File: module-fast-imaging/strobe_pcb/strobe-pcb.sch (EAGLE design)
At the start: 7 parts, among them IC2 PIC16F18857

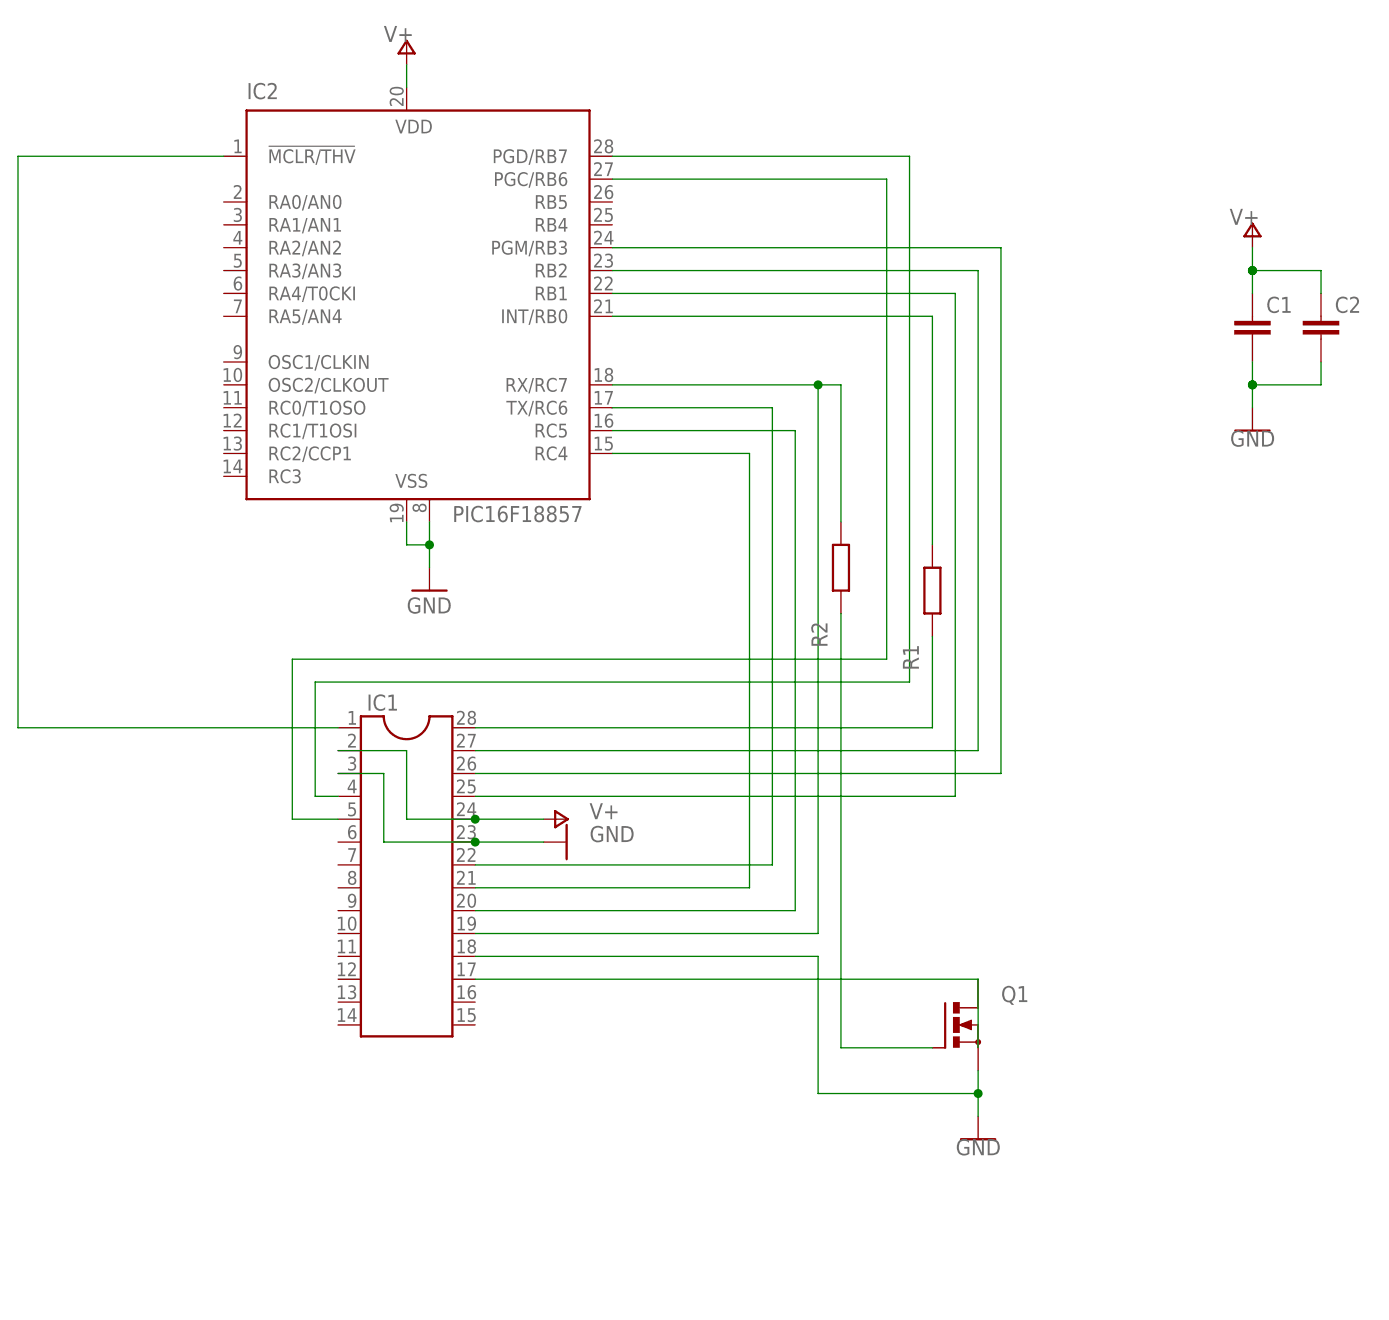
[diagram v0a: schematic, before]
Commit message: First strobe PCB submitted.
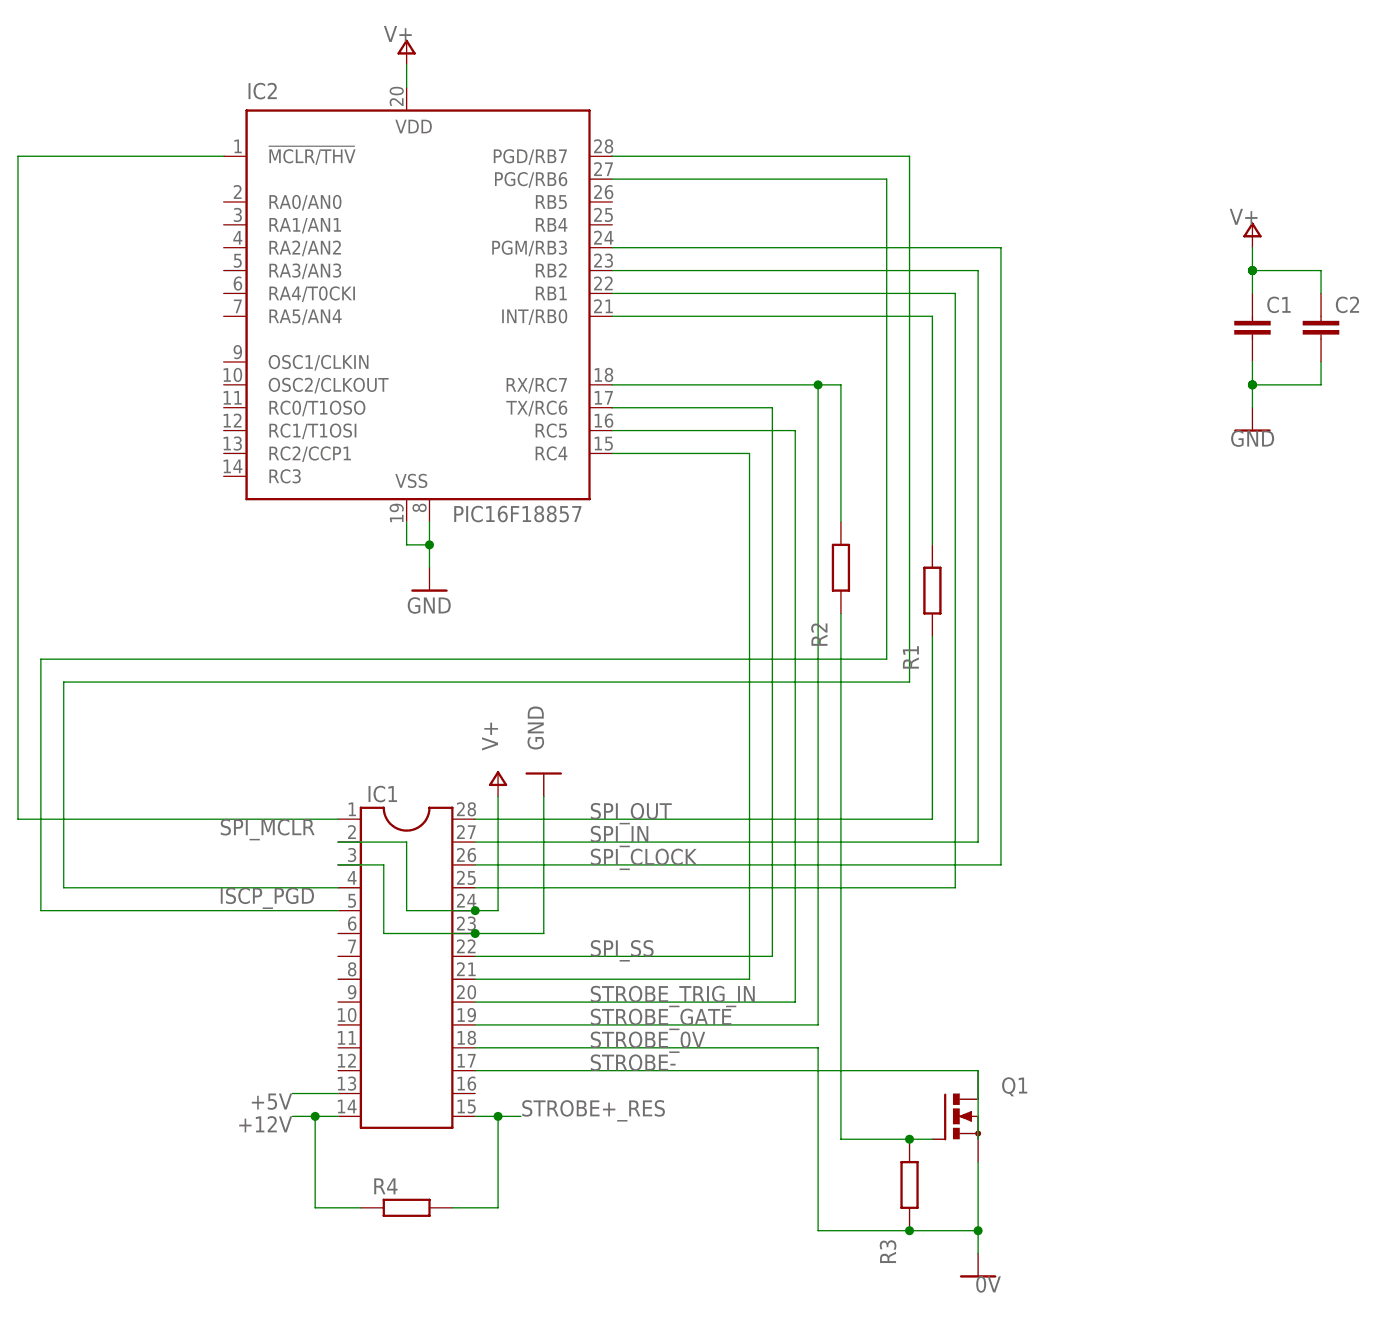
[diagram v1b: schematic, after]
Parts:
- added R3: (no value), rcl:R-EU_R1206
- added R4: (no value), rcl:R-EU_0207/10
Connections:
- net N$10 renamed SPI_IN
- net N$11 renamed STROBE_GATE
- net N$13 renamed SPI_SS
- net N$15 renamed STROBE_TRIG_IN
- net N$3 renamed SPI_OUT
- net N$4 renamed SPI_CLOCK
- net N$5 renamed SPI_MCLR
- net N$9 renamed ISCP_PGD
- net V_HIGH renamed STROBE-
- new net +12V: IC1.14, R4.1
- new net +5V: IC1.13
- new net STROBE+_RES: IC1.15, R4.2
- new net STROBE_0V: IC1.18, Q1.S, R3.1
- net GND: no longer IC1.18, Q1.S
- net N$12: now also R3.2
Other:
- moved on the sheet: IC1, Q1
